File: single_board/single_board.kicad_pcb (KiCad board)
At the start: 4 copper layers, 100 x 100 mm, 126 parts, among them J11 SPI Debug, J17 BOOTSEL, J2 USB_C_Receptacle_USB2.0_16P, J3 SWD, J30 JST_GH_H, J31 JST_GH_H, J33 JST_GH_H, J34 PB_Vertical, J35 JST_GH_H, J36 JST_GH_H, J37 JST_GH_H, J38 PB_Vertical, J39 PB_Vertical, J40 PB_Vertical, J41 PB_Vertical, J42 PB_Vertical, J43 PB_Vertical, J44 PB_Vertical, J45 PB_Vertical, J46 PB_Vertical, J47 PB_Vertical, J48 PB_Vertical, J49 PB_Vertical, J5 JST-GH, J50 PB_Vertical, J53 PB_Vertical, J55 PB_Vertical, J56 Power, J57 PB_Vertical, J6 JST-GH, Q1 AO3400A, Q3 AO3401A, SW1 Button, U1 AP2112K-3.3, U3 USBLC6-2SC6, U4 LSM6DSV, U5 STM32G474VBTx, Y2 ABM8-16MHz

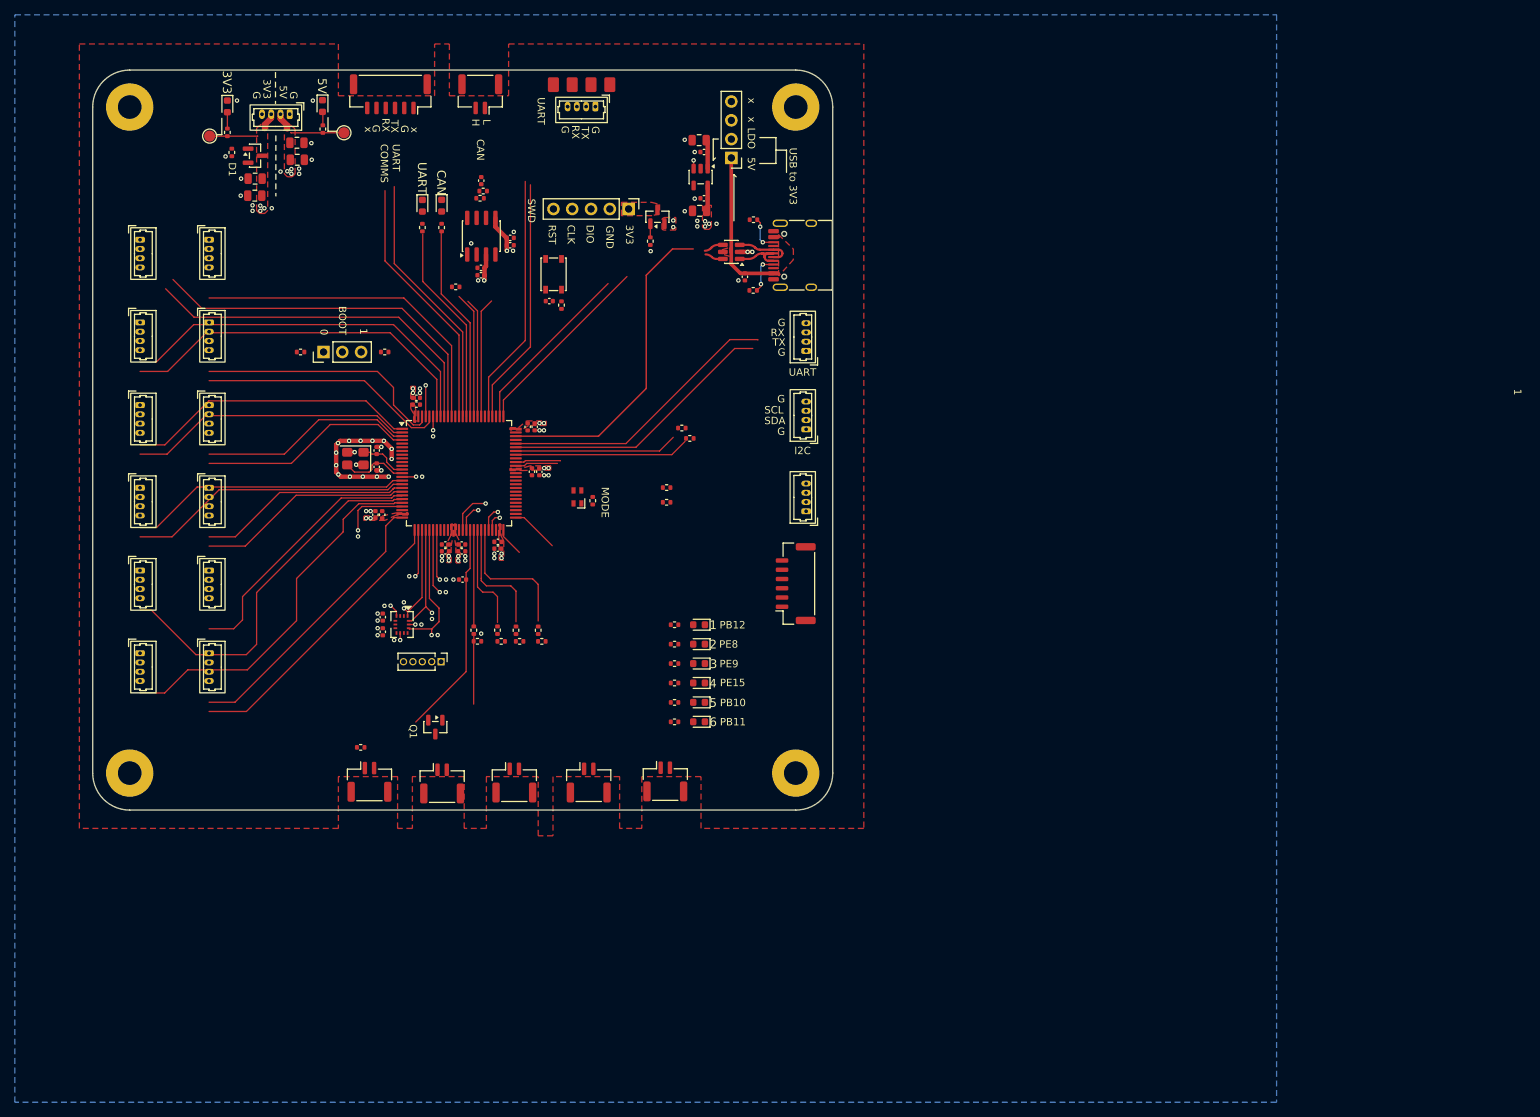
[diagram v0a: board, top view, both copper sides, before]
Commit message: Arm Motor Silkscreen
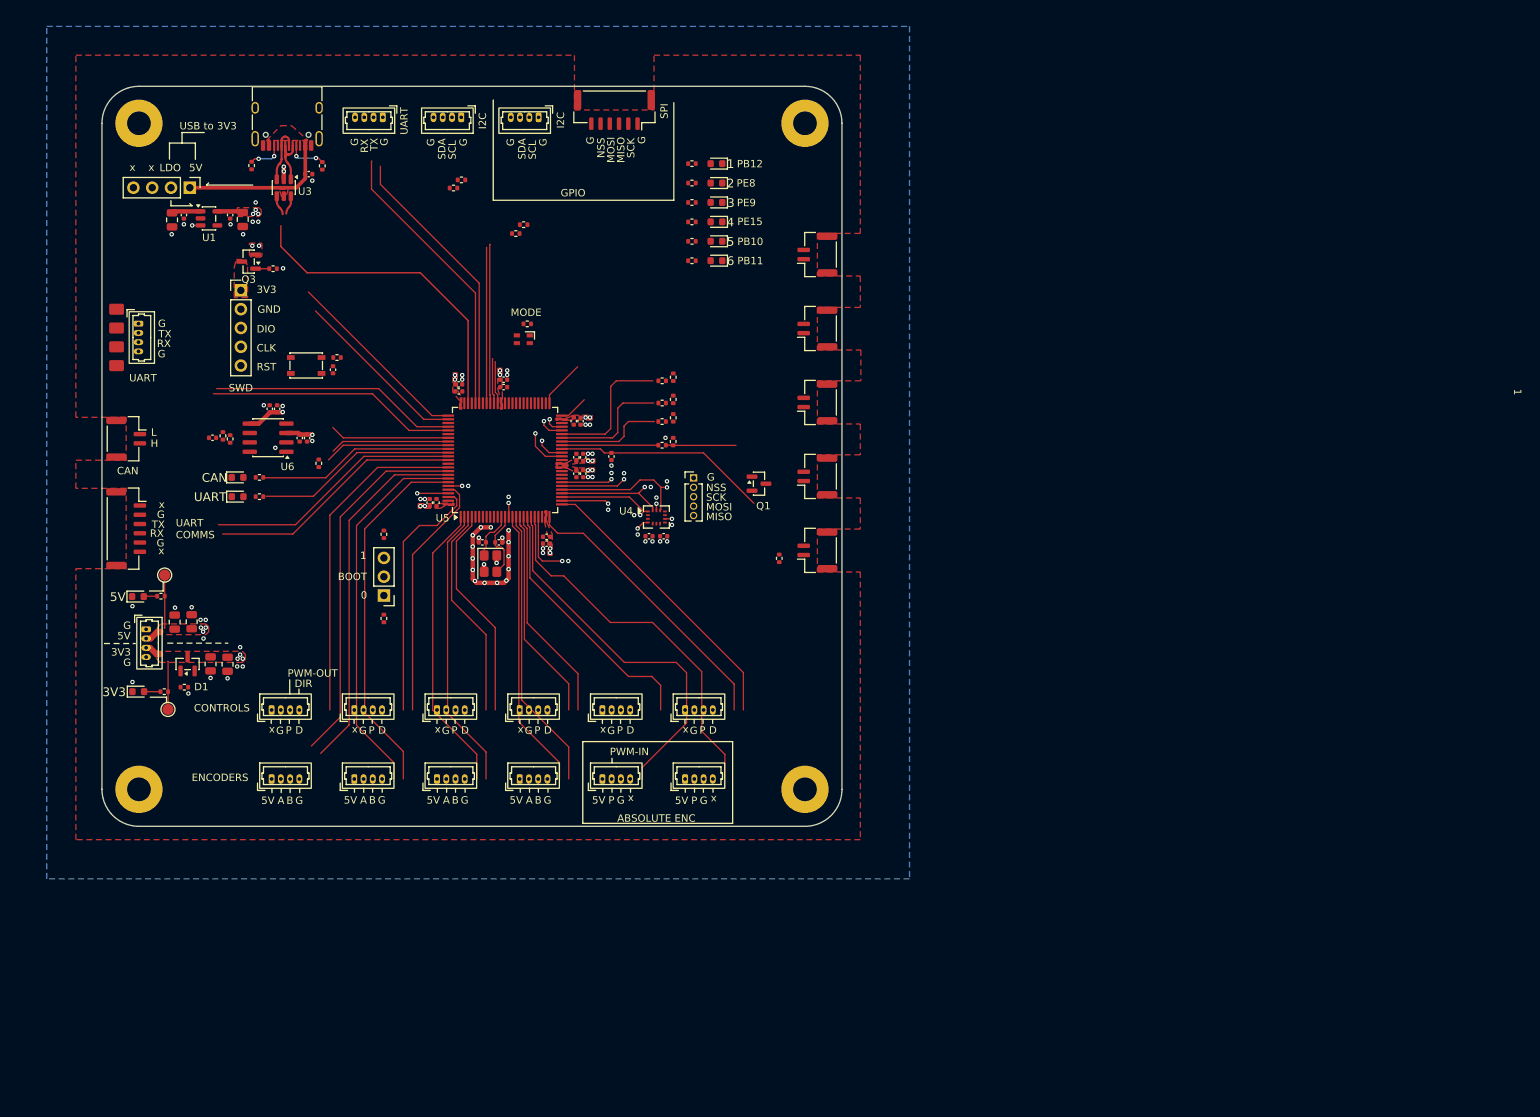
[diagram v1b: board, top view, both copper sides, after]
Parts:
- moved H1 92.2 mm to (52.0, 122.7), turned to 90 degrees
- moved H2 91.3 mm to (142.1, 122.7), turned to 90 degrees
- moved H3 88.8 mm to (52.0, 32.7), turned to 90 degrees
- moved H4 87.8 mm to (142.1, 32.7), turned to 90 degrees
- moved D4 80.0 mm to (52.0, 109.5), turned to 0 degrees
- moved TP2 77.7 mm to (56.0, 111.9), turned to 0 degrees
- moved R15 76.0 mm to (55.5, 109.5), turned to 180 degrees
- moved J43 75.6 mm to (125.8, 121.3), turned to 0 degrees
- moved J39 75.0 mm to (70.0, 121.3), turned to 0 degrees
- moved J33 74.1 mm to (143.7, 50.5), turned to 90 degrees
- moved J56 73.3 mm to (58.9, 41.4), turned to -90 degrees
- moved J54 73.0 mm to (47.0, 65.5), turned to 90 degrees
- moved R37 72.5 mm to (58.2, 108.9), turned to 0 degrees
- moved J2 72.3 mm to (72.1, 31.7), turned to 180 degrees
- moved J34 72.3 mm to (53.0, 101.1), turned to -90 degrees
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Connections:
- J50 pad 2: /I2C3_SDA -> /I2C3_SCL
- J50 pad 3: /I2C3_SCL -> /I2C3_SDA
- J57 pad 2: /I2C4_SDA -> /I2C4_SCL
- J57 pad 3: /I2C4_SCL -> /I2C4_SDA
- R5 pad 2: /I2C3_SDA -> /I2C3_SCL
- R7 pad 2: /I2C4_SDA -> /I2C4_SCL
- R8 pad 2: /I2C3_SCL -> /I2C3_SDA
- R9 pad 2: /I2C4_SCL -> /I2C4_SDA
- U5 pad 67: unconnected-(U5-PC8-Pad67) -> /I2C3_SCL
- U5 pad 69: /I2C3_SCL -> unconnected-(U5-PA8-Pad69)
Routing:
- net /I2C3_SDA: track 23.6 -> 21.1 mm
- net /I2C3_SCL: track 22.0 -> 21.5 mm
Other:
- board text added: "A"
- board text added: "ABSOLUTE ENC"
- board text added: "B"
- board text added: "CONTROLS"
- board text added: "D"
- board text added: "DIR"
- board text added: "ENCODERS"
- board text added: "GPIO"
- board text added: "MISO"
- board text added: "MOSI"
- board text added: "NSS"
- board text added: "P"
- board text added: "PWM-IN"
- board text added: "PWM-OUT"
- board text added: "SCK"
- board text added: "SPI"
